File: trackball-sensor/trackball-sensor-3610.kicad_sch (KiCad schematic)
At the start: 14 parts, among them J1 SM06B-SRSS-TB(LF)(SN), U1 PMW3360DM-T2QU, U2 TLV74318PDBVR

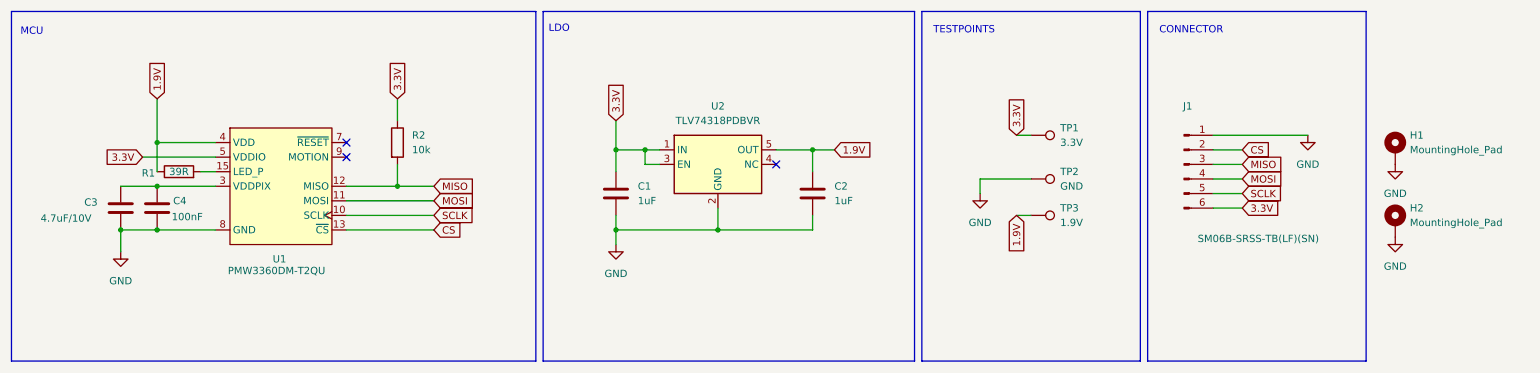
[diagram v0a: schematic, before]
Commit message: Adding 3610
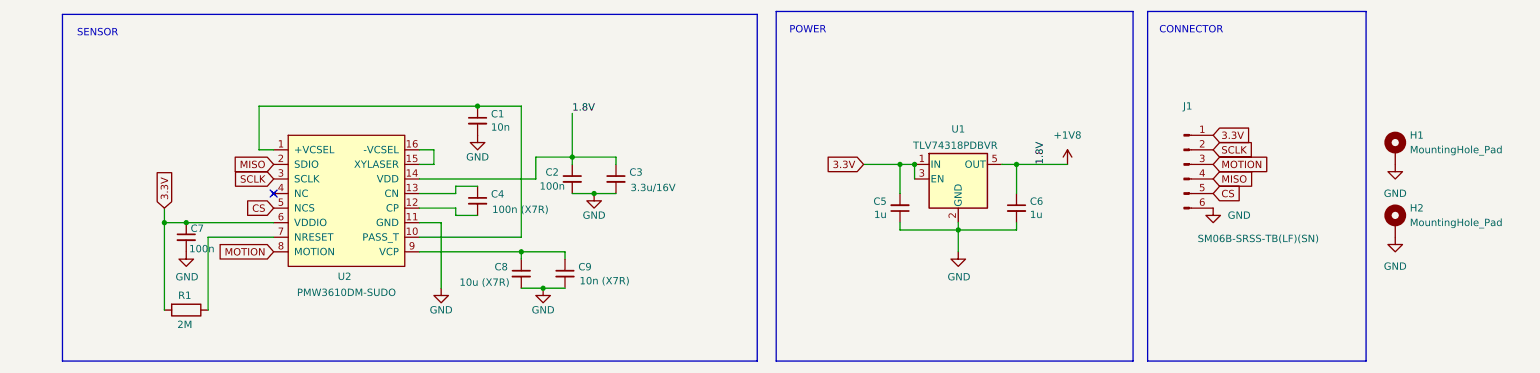
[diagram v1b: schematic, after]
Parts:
- removed C1, C2: 1uF, Capacitor_SMD:C_0402_1005Metric, symbol Device:C
- removed C3: 4.7uF/10V, Capacitor_SMD:C_0402_1005Metric, symbol Device:C
- removed C4: 100nF, Capacitor_SMD:C_0402_1005Metric, symbol Device:C
- removed R2: 10k, PCM_Resistor_SMD_AKL:R_0402_1005Metric, symbol Device:R
- removed TP1: 3.3V, TestPoint:TestPoint_Pad_D1.5mm, symbol Connector:TestPoint
- removed TP2: GND, TestPoint:TestPoint_Pad_D1.5mm, symbol Connector:TestPoint
- removed TP3: 1.9V, TestPoint:TestPoint_Pad_D1.5mm, symbol Connector:TestPoint
- removed U1: PMW3360DM-T2QU, PCM_pmw3360_pcb:PMW3360DM-T2QU 16Pin, symbol PCM_pmw3360_pcb:PMW3360DM-T2QU
- removed U2: TLV74318PDBVR, Package_TO_SOT_SMD:SOT-23-5, symbol PCM_pmw3360_pcb:TLV74318PDBVR
- added C1: 10n, Capacitor_SMD:C_0603_1608Metric, symbol Device:C_Small
- added C2, C7: 100n, Capacitor_SMD:C_0603_1608Metric, symbol Device:C_Small
- added C3: 3.3u/16V, Capacitor_SMD:C_0603_1608Metric, symbol Device:C_Small
- added C4: 100n (X7R), Capacitor_SMD:C_0603_1608Metric, symbol Device:C_Small
- added C5, C6: 1u, Capacitor_SMD:C_0603_1608Metric, symbol Device:C_Small
- added C8: 10u (X7R), Capacitor_SMD:C_0603_1608Metric, symbol Device:C_Small
- added C9: 10n (X7R), Capacitor_SMD:C_0603_1608Metric, symbol Device:C_Small
- added U1: TLV74318PDBVR, Package_TO_SOT_SMD:SOT-23-5, symbol Regulator_Linear:TLV70218_SOT23-5
- added U2: PMW3610DM-SUDO, PMW3610:PMW3610DM-SUDU 16Pin, symbol mysymbol:PMW3610
- J1: footprint PCM_marbastlib-xp-various:SM06B-SRSS-TB(LF)(SN) -> Connector_JST:JST_SH_SM06B-SRSS-TB_1x06-1MP_P1.00mm_Horizontal
- R1: value 39R -> 2M; footprint PCM_Resistor_SMD_AKL:R_0402_1005Metric -> Resistor_SMD:R_0603_1608Metric; LCSC (none) -> C22976
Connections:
- net MOSI is gone; now on net MISO: J1.4 (Pin_4)
- net 3.3V: now also J1.1 (Pin_1), R1.2, C5.2, C7.1, U1.1 (IN), U1.3 (EN), U2.6 (VDDIO); no longer J1.6 (Pin_6)
- net CS: now also J1.5 (Pin_5), U2.5 (NCS); no longer J1.2 (Pin_2)
- net GND: now also J1.6 (Pin_6), C1.2, C2.2, C3.2, C5.1, C6.2, C7.2, C8.2, C9.2, U1.2 (GND), U2.11 (GND); no longer J1.1 (Pin_1)
- net MISO: now also U2.2 (SDIO); no longer J1.3 (Pin_3)
- net SCLK: now also J1.2 (Pin_2), U2.3 (SCLK); no longer J1.5 (Pin_5)
- net 1.9V: no longer names the net of R1.1
- net 1.9V: now also U2.7 (NRESET)
- new net: C8.1, C9.1, U2.9 (VCP)
- new net: C1.1, U2.1 (+VCSEL), U2.10 (PASS_T)
- new net: C4.2, U2.12 (CP)
- new net: C4.1, U2.13 (CN)
- new net: U2.15 (XYLASER), U2.16 (-VCSEL)
- new net +1V8: C2.1, C3.1, C6.1, U1.5 (OUT), U2.14 (VDD)
- new net MOTION: J1.3 (Pin_3), U2.8 (MOTION)
- no-connect marks 3 -> 1
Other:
- note added: "POWER"
- note added: "SENSOR"
- note removed: "LDO"
- note removed: "MCU"
- note removed: "TESTPOINTS"
